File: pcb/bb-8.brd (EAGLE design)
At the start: 128.3 x 50.8 mm, 24 parts, among them T1 2N2222, X1 STEREOJACK

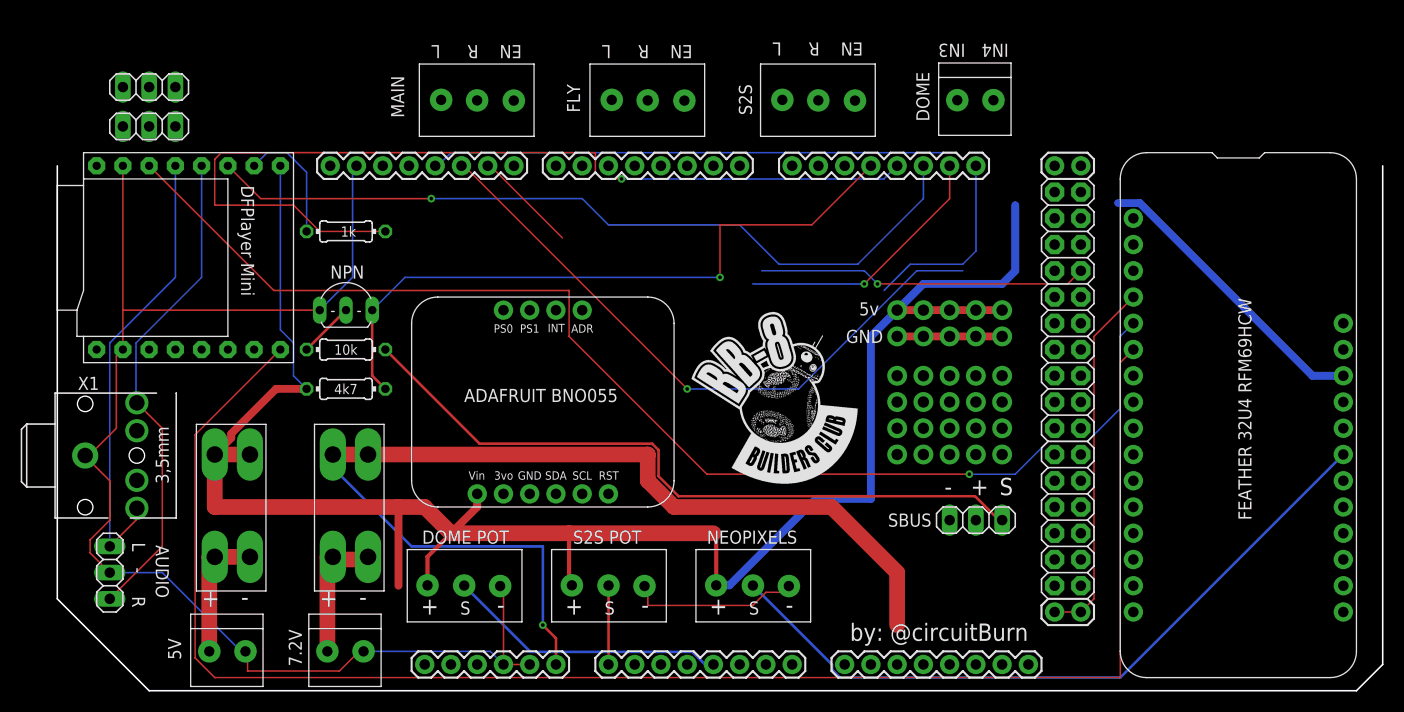
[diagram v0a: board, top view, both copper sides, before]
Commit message: Squashed commit of the following:
commit c327650e5103bb6a6949c6a1538a163dea4dba5a
Author: Patrick Ryan <pat.m.ryan@gmail.com>
Date:   Sat Aug 20 09:49:49 2022 -0400

    Updates to PCB

commit 971e034c2edcb3dc5db781baa092387508605f21
Author: Patrick Ryan <pat.m.ryan@gmail.com>
Date:   Sat Aug 20 09:49:32 2022 -0400

    Splitting up main drive into separate files

commit 5c3a9991173692b4d5a5e5dc78048e5e86c772e9
Author: Patrick Ryan <pat.m.ryan@gmail.com>
Date:   Fri Jul 1 13:35:34 2022 -0400

    Splitting up drive functions into separate files
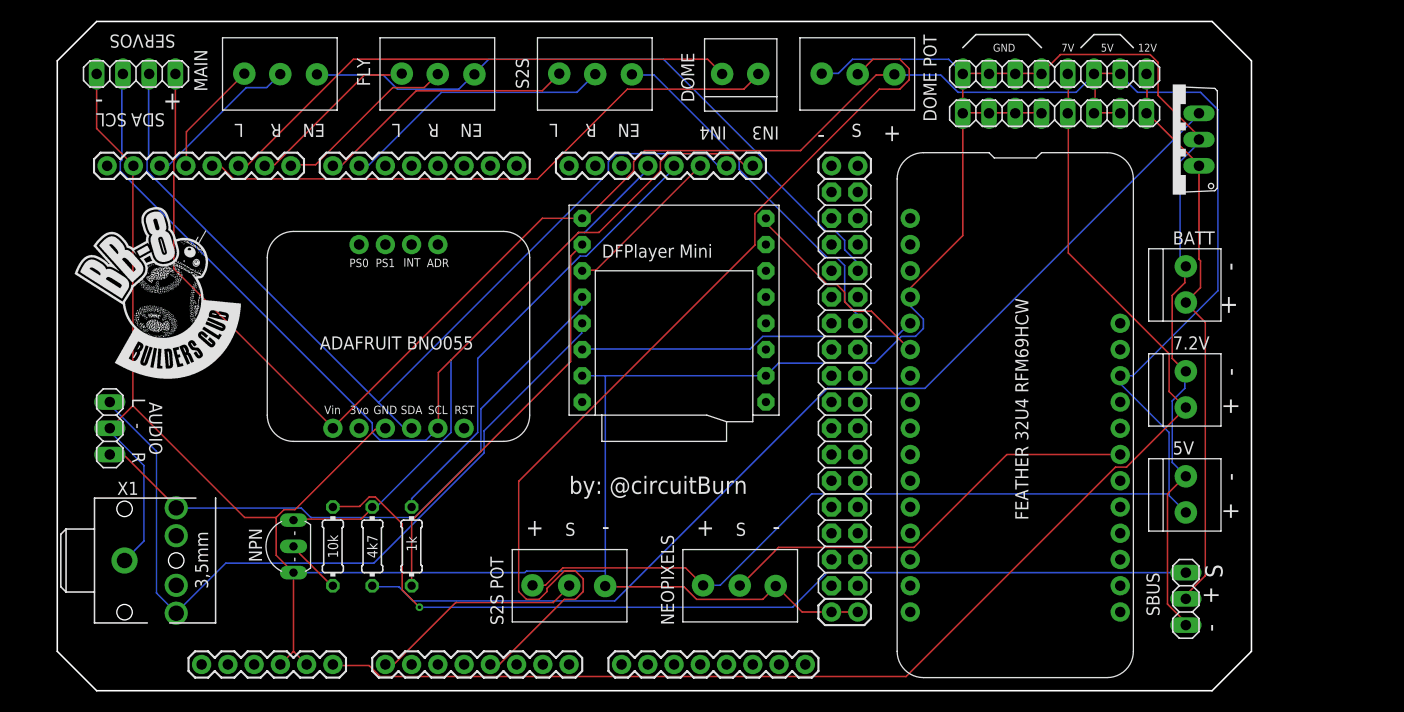
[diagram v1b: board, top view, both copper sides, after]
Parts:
- removed 7.2V: 1X2-3.5MM, adafruit:1X2-3.5MM
- removed SERVO1, SERVO2: (no value), pinhead:1X03
- removed U$4, U$5: KEYSTONE_3568, BB8:KEYSTONE_3568
- added 12V, 7V2: 1X2-3.5MM, adafruit:1X2-3.5MM
- added IC1: 786TV, linear:TO220V
- added JP2: (no value), pinhead:1X04
- added JP3, JP4: (no value), pinhead:1X08
- moved 5V 94.0 mm to (109.2, 19.1), turned to 270 degrees
- moved DOME_POT 62.5 mm to (77.5, 59.7), turned to 180 degrees
- moved U$1 47.3 mm to (59.7, 36.8), turned to 0 degrees
- moved R3 31.1 mm to (34.3, 14.0), turned to 270 degrees
- moved T1 25.0 mm to (21.6, 14.0), turned to 90 degrees
- moved DOME 23.0 mm to (66.0, 59.7), turned to 0 degrees
- moved S2S 21.7 mm to (52.1, 59.7)
- moved SBUS 21.7 mm to (109.2, 8.89), turned to 90 degrees
- moved U$3 21.6 mm to (81.3, 52.1)
- moved U$7 21.6 mm to (30.5, 26.7)
- moved FLY 20.5 mm to (36.8, 59.7)
- moved MAIN 19.2 mm to (21.6, 59.7)
- moved R1 19.1 mm to (26.7, 14.0), turned to 270 degrees
- moved R2 15.5 mm to (30.5, 14.0), turned to 270 degrees
- moved U$2 15.3 mm to (20.3, 24.1)
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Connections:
- removed net N$20: 5V.1, U$4.2A
- removed net N$21: 7.2V.1, U$5.2A
- new net +12V: 12V.1, IC1.1, JP3.1, JP4.1, SBUS.2
- new net 5V_RAW: IC1.3, R2.2
- net +5V: now also 5V.1, JP2.1, JP3.2, JP3.3, JP4.2, JP4.3; no longer R2.2, SBUS.2, U$4.1A
- net +7V: now also 7V2.1, JP3.4, JP4.4; no longer SERVO1.2, SERVO2.2, U$5.1A
- net GND: now also 12V.2, 7V2.2, IC1.2, JP2.4, JP3.5, JP3.6, JP3.7, JP3.8, JP4.5, JP4.6, JP4.7, JP4.8; no longer 7.2V.2, SERVO1.3, SERVO2.3
- net SCL: now also JP2.3
- net SDA: now also JP2.2
- net SERVO_1: no longer SERVO1.1
- net SERVO_2: no longer SERVO2.1
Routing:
- net GND: track 196.5 -> 344.4 mm, vias 1 -> 0
- net BUSY: track 155.9 -> 20.0 mm
- net 5V_RAW: track 0.00 -> 100.3 mm
- net SPK: track 120.4 -> 32.8 mm, vias 1 -> 0
- net SCL: track 18.7 -> 97.7 mm
- net DOME_POT: track 27.3 -> 94.7 mm
- net SDA: track 25.6 -> 90.2 mm, vias 1 -> 0
- net RX1: track 77.1 -> 15.6 mm, vias 1 -> 0
- net +5V: track 207.2 -> 263.4 mm
- net +12V: track 0.00 -> 55.2 mm
- net TX1: track 91.0 -> 43.9 mm, vias 1 -> 0
- net S2S_EN: track 0.65 -> 34.9 mm
- net MAIN_EN: track 31.9 -> 64.2 mm, vias 1 -> 0
- net N$6: track 44.2 -> 75.8 mm
- net +7V: track 102.6 -> 131.0 mm, vias 1 -> 0
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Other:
- board size 128.3 x 50.8 mm -> 115.6 x 64.8 mm
- board text added: "12V"
- board text added: "5V"
- board text added: "7.2V"
- board text added: "7V"
- board text added: "BATT"
- board text added: "SCL"
- board text added: "SDA"
- board text added: "SERVOS"
- board text removed: "5v"

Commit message: Updates to board
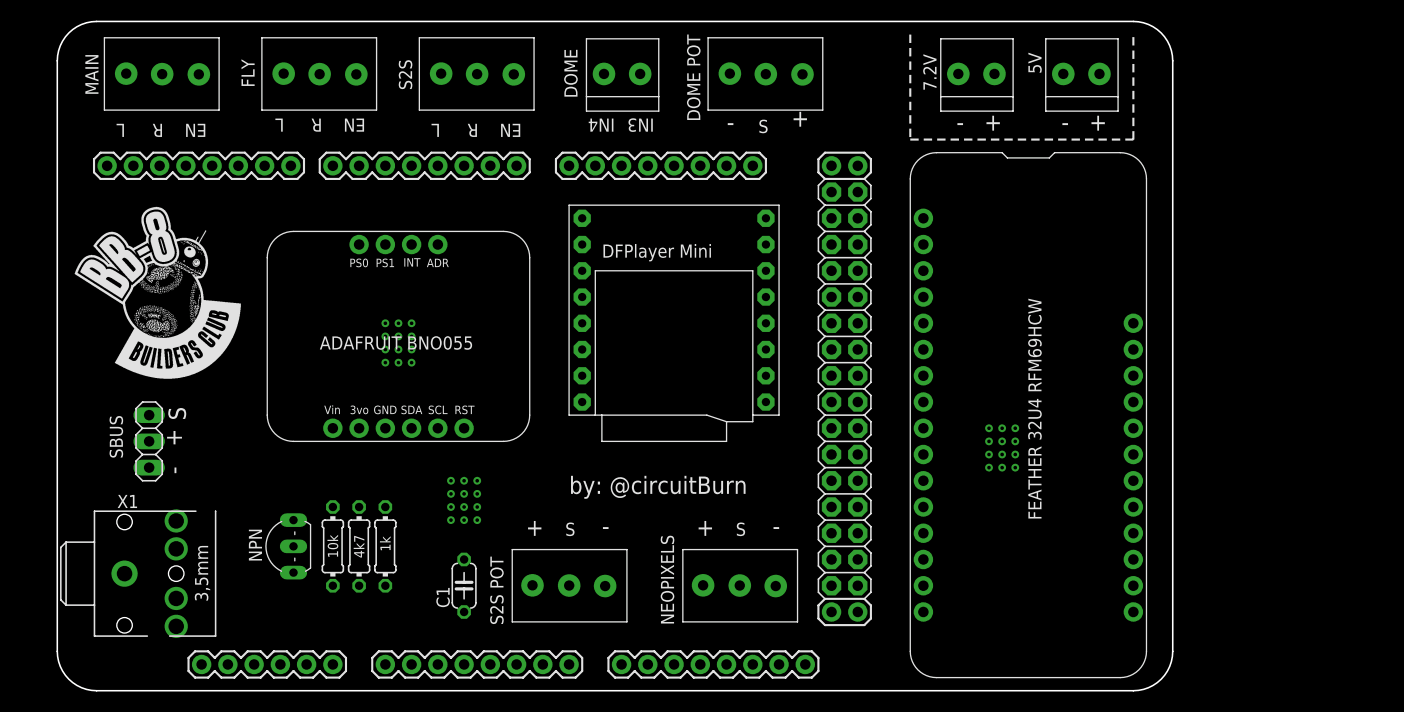
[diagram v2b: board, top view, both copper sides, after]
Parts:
- removed 12V: 1X2-3.5MM, adafruit:1X2-3.5MM
- removed IC1: 786TV, linear:TO220V
- removed JP1: (no value), pinhead:1X03
- removed JP2: (no value), pinhead:1X04
- removed JP3, JP4: (no value), pinhead:1X08
- added C1: 0.22uF, rcl:C050-024X044
- moved SBUS 101.5 mm to (8.89, 24.1)
- moved 5V 41.9 mm to (99.1, 59.7), turned to 0 degrees
- moved 7V2 36.6 mm to (88.9, 59.7), turned to 0 degrees
- moved DOME 11.4 mm to (54.6, 59.7)
- moved FLY 11.4 mm to (25.4, 59.7)
- moved MAIN 11.4 mm to (10.2, 59.7)
- moved S2S 11.4 mm to (40.6, 59.7)
- moved DOME_POT 8.89 mm to (68.6, 59.7)
- moved R3 2.54 mm to (31.8, 14.0)
- moved R2 1.27 mm to (29.2, 14.0)
- moved X1 1.27 mm to (3.81, 11.4)
- moved U$3 1.27 mm to (82.5, 52.1)
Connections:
- removed net +12V: 12V.1, IC1.1, JP3.1, JP4.1, SBUS.2
- removed net 5V_RAW: IC1.3, R2.2
- removed net SERVO_1: U$7.5
- removed net SERVO_2: U$7.4
- net +5V: now also R2.2; no longer JP2.1, JP3.2, JP3.3, JP4.2, JP4.3
- net +7V: now also SBUS.2; no longer JP3.4, JP4.4
- net DAC_R: no longer JP1.3
- net GND: now also C1.2; no longer 12V.2, IC1.2, JP1.2, JP2.4, JP3.5, JP3.6, JP3.7, JP3.8, JP4.5, JP4.6, JP4.7, JP4.8
- net N$6: no longer JP1.1
- net S2S_POT: now also C1.1
- net SCL: no longer JP2.3
- net SDA: no longer JP2.2
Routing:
- net GND: track 344.4 -> 0.00 mm
- net +5V: track 263.4 -> 0.00 mm
- net +7V: track 131.0 -> 0.00 mm
- net 5V_RAW: track 100.3 -> 0.00 mm
- net SCL: track 97.7 -> 0.00 mm
- net DOME_POT: track 94.7 -> 0.00 mm
- net N$5: track 92.5 -> 0.00 mm, vias 1 -> 0
- net SDA: track 90.2 -> 0.00 mm
- net N$6: track 75.8 -> 0.00 mm
- net MAIN_EN: track 64.2 -> 0.00 mm
- net DAC_R: track 60.1 -> 0.00 mm
- net IN3: track 57.6 -> 0.00 mm
- net +12V: track 55.2 -> 0.00 mm
- net SBUS: track 53.0 -> 0.00 mm
- net IN4: track 51.7 -> 0.00 mm
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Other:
- board size 115.6 x 64.8 mm -> 108 x 64.8 mm
- board text removed: "12V"
- board text removed: "7V"
- board text removed: "AUDIO"
- board text removed: "BATT"
- board text removed: "GND"
- board text removed: "SCL"
- board text removed: "SDA"
- board text removed: "SERVOS"
